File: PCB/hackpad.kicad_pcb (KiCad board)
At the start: 2 copper layers, 76.5 x 110.5 mm, 27 parts, among them SW1 SW_Push, SW10 RotaryEncoder_Switch, SW11 SW_Push, SW12 SW_Push, SW13 SW_Push, SW14 SW_Push, SW15 SW_Push, SW16 SW_Push, SW17 SW_Push, SW2 SW_Push, SW3 SW_Push, SW4 SW_Push, SW5 SW_Push, SW6 SW_Push, SW7 SW_Push, SW8 SW_Push, SW9 SW_Push, U1 MOUDLE-SEEEDUINO-XIAO, U2 MCP23017x-x-SO

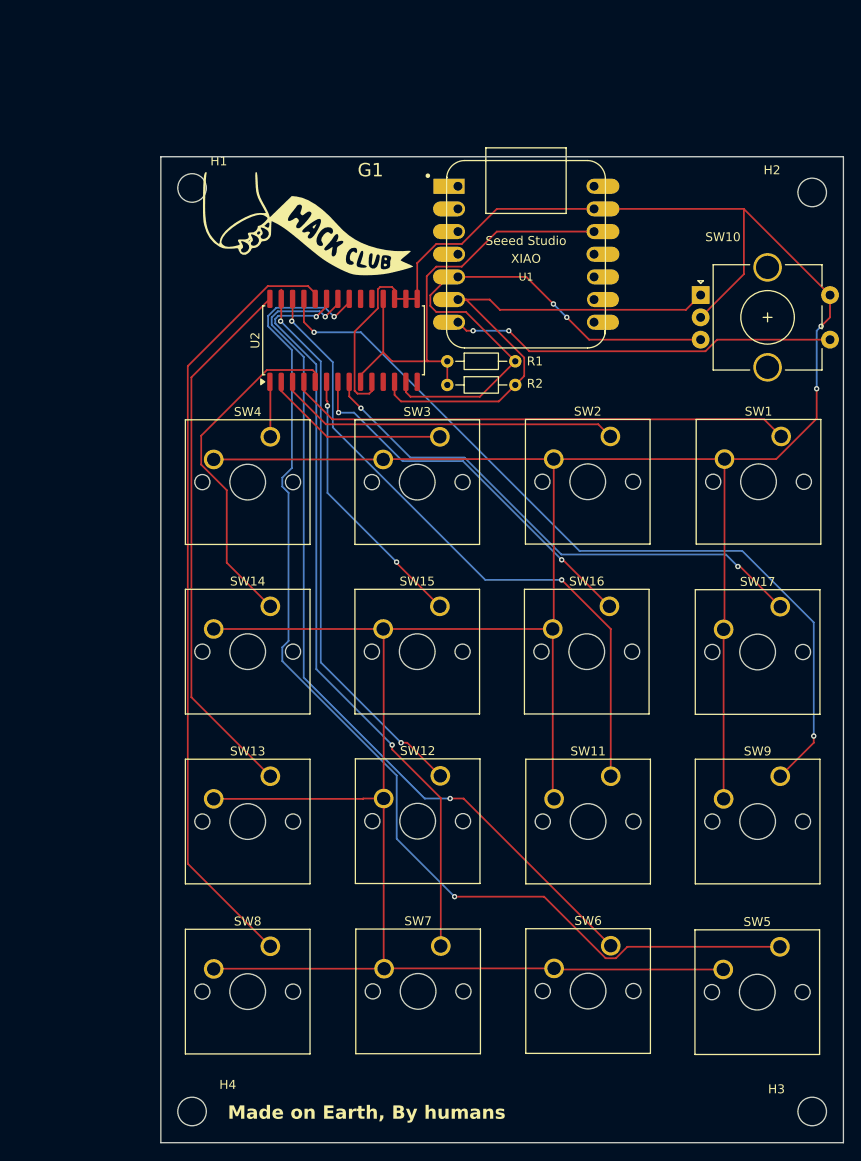
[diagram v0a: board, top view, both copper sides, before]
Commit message: Diode matrix
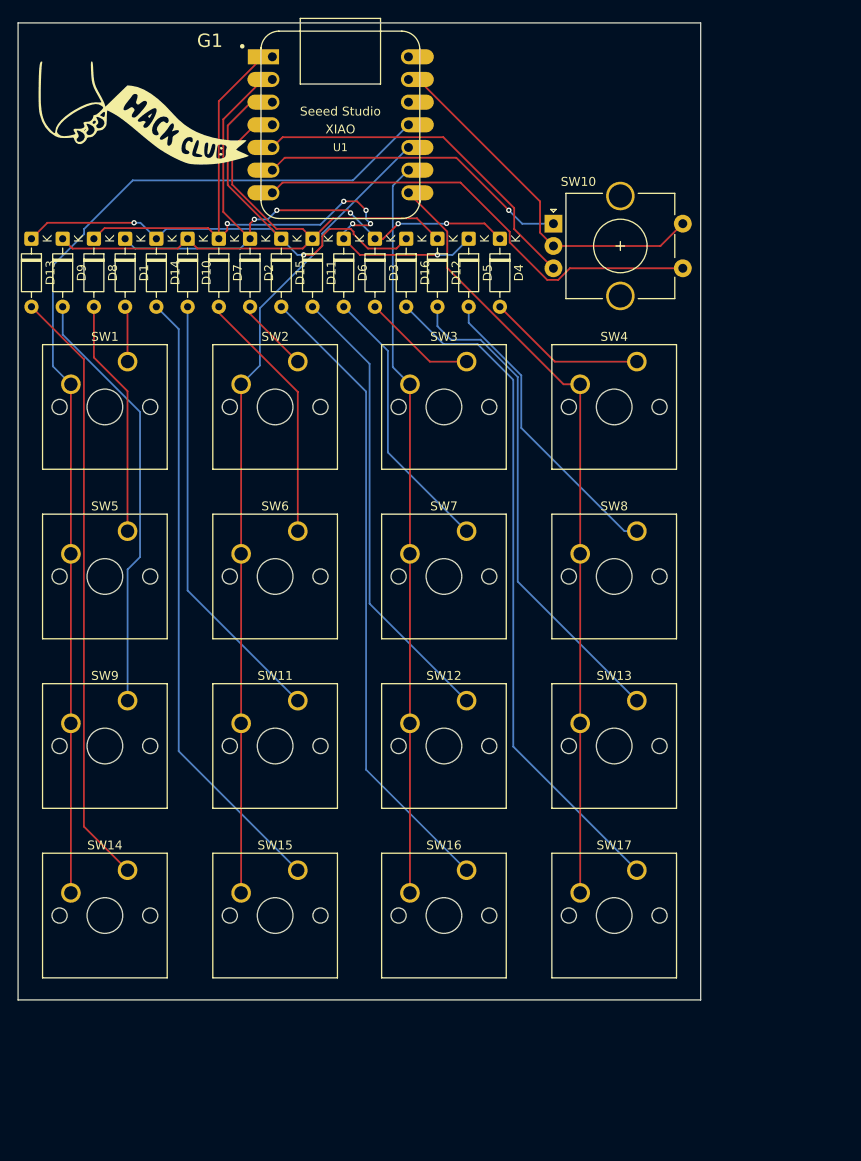
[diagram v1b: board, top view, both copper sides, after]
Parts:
- removed H1, H2, H3, H4: MountingHole_3.2mm_M3, MountingHole:MountingHole_3.2mm_M3
- removed R1, R2: 4.7K, Resistor_THT:R_Axial_DIN0204_L3.6mm_D1.6mm_P7.62mm_Horizontal
- removed U2: MCP23017x-x-SO, Package_SO:SOIC-28W_7.5x17.9mm_P1.27mm
- added D1: D, Diode_THT:D_DO-35_SOD27_P7.62mm_Horizontal, F.Cu at (101.0, 52.7)
- added D10: D, Diode_THT:D_DO-35_SOD27_P7.62mm_Horizontal, F.Cu at (108.0, 52.7)
- added D11: D, Diode_THT:D_DO-35_SOD27_P7.62mm_Horizontal, F.Cu at (122.0, 52.7)
- added D12: D, Diode_THT:D_DO-35_SOD27_P7.62mm_Horizontal, F.Cu at (136.0, 52.7)
- added D13: D, Diode_THT:D_DO-35_SOD27_P7.62mm_Horizontal, F.Cu at (90.5, 52.7)
- added D14: D, Diode_THT:D_DO-35_SOD27_P7.62mm_Horizontal, F.Cu at (104.5, 52.7)
- added D15: D, Diode_THT:D_DO-35_SOD27_P7.62mm_Horizontal, F.Cu at (118.5, 52.7)
- added D16: D, Diode_THT:D_DO-35_SOD27_P7.62mm_Horizontal, F.Cu at (132.5, 52.7)
- added D2: D, Diode_THT:D_DO-35_SOD27_P7.62mm_Horizontal, F.Cu at (115.0, 52.7)
- added D3: D, Diode_THT:D_DO-35_SOD27_P7.62mm_Horizontal, F.Cu at (129.0, 52.7)
- added D4: D, Diode_THT:D_DO-35_SOD27_P7.62mm_Horizontal, F.Cu at (143.0, 52.7)
- added D5: D, Diode_THT:D_DO-35_SOD27_P7.62mm_Horizontal, F.Cu at (139.5, 52.7)
- added D6: D, Diode_THT:D_DO-35_SOD27_P7.62mm_Horizontal, F.Cu at (125.5, 52.7)
- added D7: D, Diode_THT:D_DO-35_SOD27_P7.62mm_Horizontal, F.Cu at (111.5, 52.7)
- added D8: D, Diode_THT:D_DO-35_SOD27_P7.62mm_Horizontal, F.Cu at (97.5, 52.7)
- added D9: D, Diode_THT:D_DO-35_SOD27_P7.62mm_Horizontal, F.Cu at (94.0, 52.7)
- moved SW5 86.7 mm to (101.3, 85.5)
- moved SW1 73.7 mm to (101.3, 66.5)
- moved SW9 73.6 mm to (101.3, 104.5)
- moved SW8 62.1 mm to (158.3, 85.5)
- moved SW6 58.2 mm to (120.3, 85.5)
- moved SW7 46.6 mm to (139.3, 85.5)
- moved SW13 41.9 mm to (158.3, 104.5)
- moved SW4 41.9 mm to (158.3, 66.5)
- moved SW11 36.1 mm to (120.3, 104.5)
- moved SW2 36.0 mm to (120.3, 66.5)
- moved SW14 33.6 mm to (101.3, 123.5)
- moved SW16 33.6 mm to (139.3, 123.5)
- moved SW17 33.6 mm to (158.3, 123.5)
- moved SW15 33.6 mm to (120.3, 123.5)
- moved U1 25.4 mm to (125.1, 39.9)
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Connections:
- net Net-(U1-PB08_A6_D6_TX) renamed TX
- SW1 pad 2: GND -> COL1
- SW11 pad 2: GND -> COL2
- SW12 pad 2: GND -> COL3
- SW13 pad 2: GND -> COL4
- SW14 pad 2: GND -> COL1
- SW15 pad 2: GND -> COL2
- SW16 pad 2: GND -> COL3
- SW17 pad 2: GND -> COL4
- SW2 pad 2: GND -> COL2
- SW3 pad 2: GND -> COL3
- SW4 pad 2: GND -> COL4
- SW5 pad 2: GND -> COL1
- SW6 pad 2: GND -> COL2
- SW7 pad 2: GND -> COL3
- SW8 pad 2: GND -> COL4
- SW9 pad 2: GND -> COL1
- U1 pad 1: unconnected-(U1-PA02_A0_D0-Pad1) -> ROW2
- U1 pad 10: unconnected-(U1-PA5_A9_D9_MISO-Pad10) -> COL2
- U1 pad 11: unconnected-(U1-PA6_A10_D10_MOSI-Pad11) -> COL1
- U1 pad 2: unconnected-(U1-PA4_A1_D1-Pad2) -> ROW1
- U1 pad 3: unconnected-(U1-PA10_A2_D2-Pad3) -> ROW4
- U1 pad 4: unconnected-(U1-PA11_A3_D3-Pad4) -> ROW3
- U1 pad 8: unconnected-(U1-PB09_A7_D7_RX-Pad8) -> COL4
- U1 pad 9: unconnected-(U1-PA7_A8_D8_SCK-Pad9) -> COL3
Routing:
- net GND: track 405.4 -> 41.6 mm, vias 2 -> 0
- net COL1: track 0.00 -> 117.9 mm
- net Net-(D8-A): track 126.0 -> 26.7 mm, vias 2 -> 0
- net COL2: track 0.00 -> 91.3 mm
- net COL4: track 0.00 -> 87.5 mm
- net COL3: track 0.00 -> 82.5 mm
- net ROW2: track 0.00 -> 79.1 mm, vias 0 -> 6
- net ROW1: track 0.00 -> 70.0 mm, vias 0 -> 5
- net ROW4: track 0.00 -> 69.8 mm, vias 0 -> 2
- net Net-(D7-A): track 97.8 -> 28.8 mm, vias 2 -> 0
- net ROW3: track 0.00 -> 66.9 mm
- net Net-(D6-A): track 85.2 -> 30.9 mm, vias 2 -> 0
- net Net-(D5-A): track 87.8 -> 33.8 mm
- net +3V3: track 51.0 -> 0.00 mm
- net Net-(D1-A): track 56.6 -> 6.26 mm
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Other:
- board size 76.5 x 110.5 mm -> 76.5 x 109.5 mm
- board text removed: "Made on Earth, By humans"
